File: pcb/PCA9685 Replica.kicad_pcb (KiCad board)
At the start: 2 copper layers, 63 x 50 mm, 63 parts, among them J1 Conn_01x03, J10 Conn_01x03, J11 Conn_01x03, J12 Conn_01x03, J13 Conn_01x03, J14 Conn_01x03, J15 Conn_01x03, J16 Conn_01x03, J17 Screw_Terminal_01x02, J18 Conn_01x06, J2 Conn_01x03, J3 Conn_01x03, J4 Conn_01x03, J5 Conn_01x03, J6 Conn_01x03, J7 Conn_01x03, J8 Conn_01x03, J9 Conn_01x03, Q1 SUD50P08-25L, U1 PCA9685PW

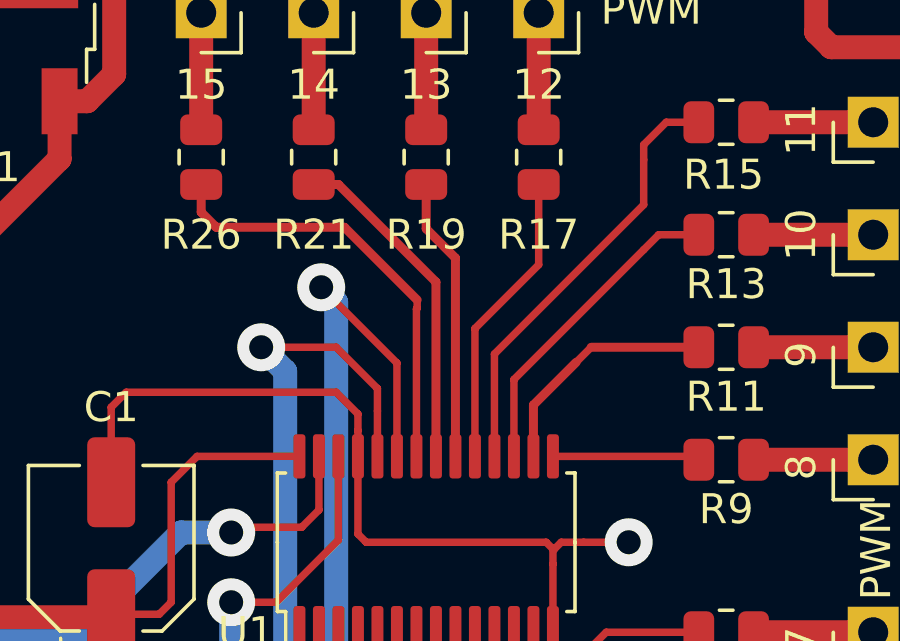
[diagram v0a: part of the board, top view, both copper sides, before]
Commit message: update pcb
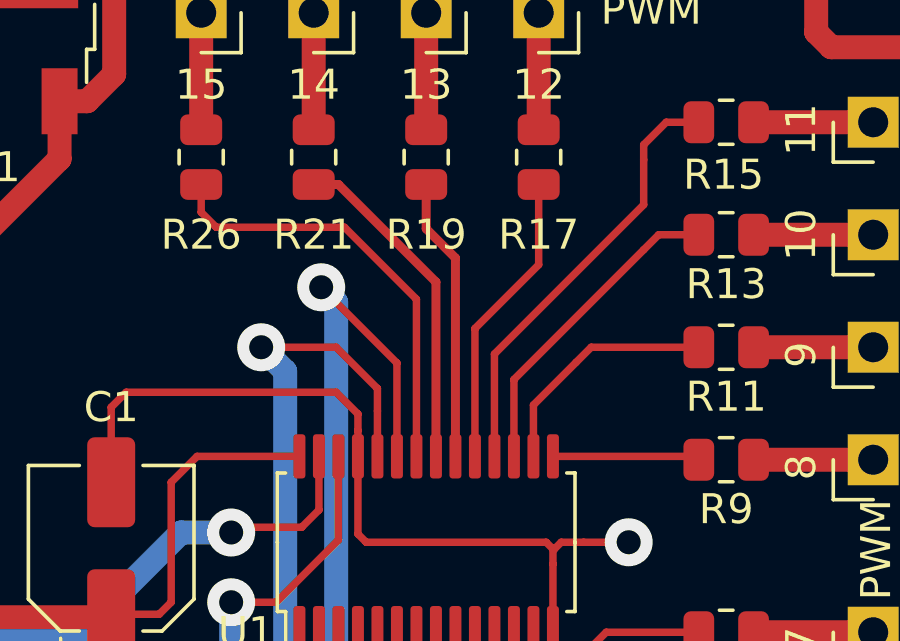
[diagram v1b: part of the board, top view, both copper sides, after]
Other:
- board text added: "Vias: - 1,6 mm / 0,8 mm - 1.4 mm / 0.7 mm"
- board text removed: "Vias: 1,6 mm / 0,8 mm"

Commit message: update
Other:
- board text added: "Minimo 10 mils Espesor de Cobre: 1oz Espesor de la tarjeta PCB: 1,6 mm Acabado Superficial: HASL"
- board text removed: "Espesor de Cobre: 1oz Espesor de la tarjeta PCB: 1,6 mm Acabado Superficial: HASL"
